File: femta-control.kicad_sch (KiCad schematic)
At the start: 13 parts, among them J2 CUBESAT INTERFACE, U4 LM358-N-Q1

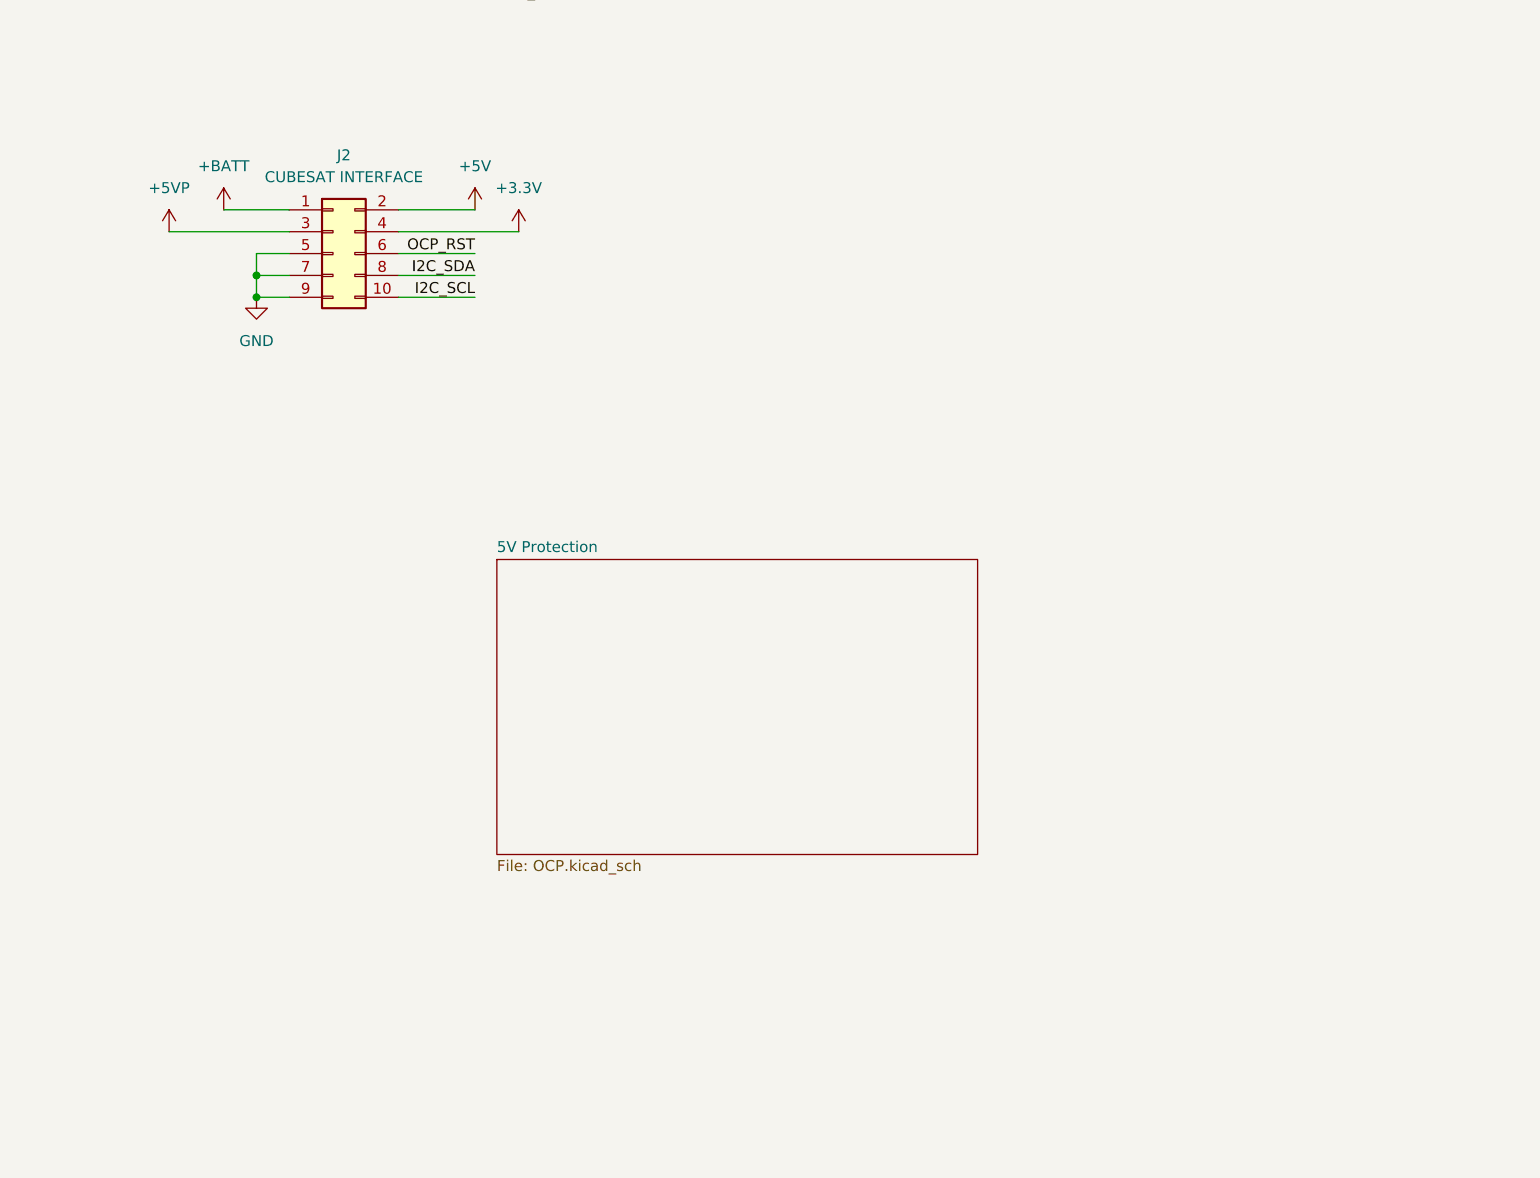
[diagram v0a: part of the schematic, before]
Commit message: ocp channels
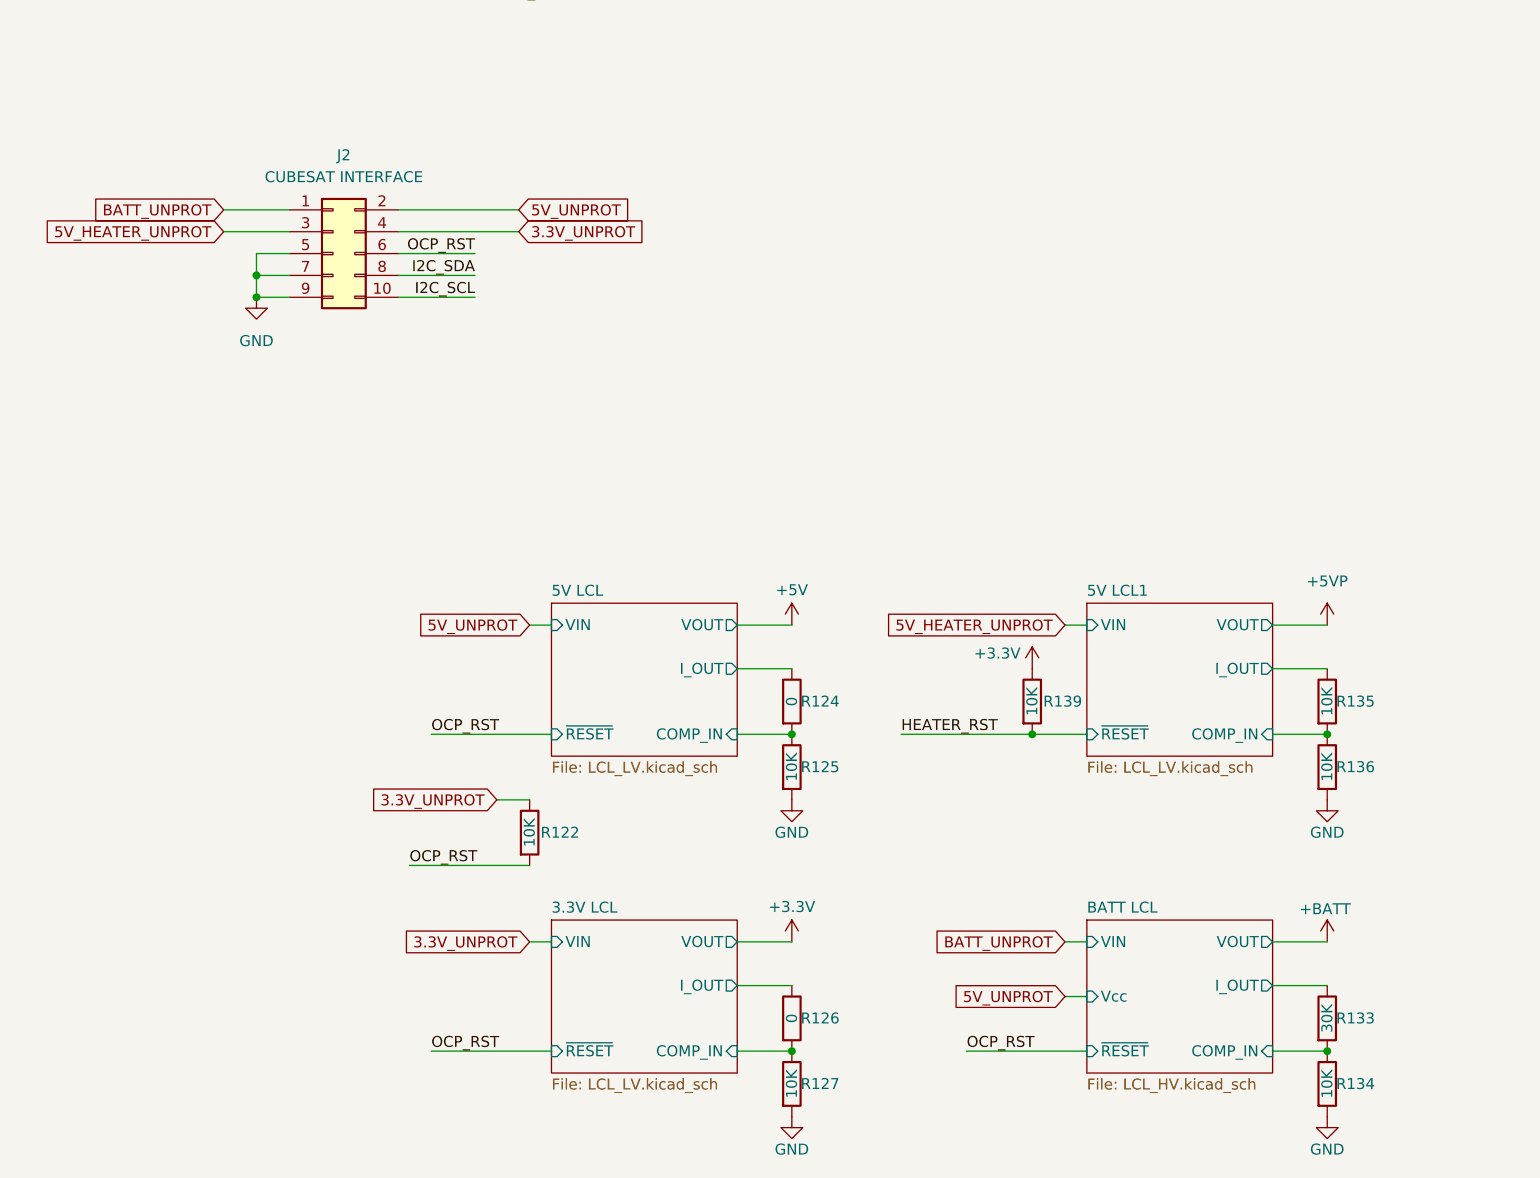
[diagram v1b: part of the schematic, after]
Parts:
- added R122, R125, R127, R134, R135, R136, R139: 10K, symbol Device:R
- added R124, R126: 0, symbol Device:R
- added R133: 30K, symbol Device:R
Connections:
- net +3.3V: now also R139.1; no longer J2.4 (Pin_4)
- net +5V: no longer J2.2 (Pin_2)
- net +5VP: no longer J2.3 (Pin_3)
- net +BATT: no longer J2.1 (Pin_1)
- net GND: now also R125.2, R127.2, R134.2, R136.2
- net OCP_RST: now also R122.2
- new net 3.3V LCL/COMP_IN: R126.2, R127.1
- new net 3.3V LCL/I_OUT: R126.1
- new net 3.3V_UNPROT: J2.4 (Pin_4), R122.1
- new net 5V LCL/COMP_IN: R124.2, R125.1
- new net 5V LCL/I_OUT: R124.1
- new net 5V LCL1/COMP_IN: R135.2, R136.1
- new net 5V LCL1/I_OUT: R135.1
- new net 5V_HEATER_UNPROT: J2.3 (Pin_3)
- new net 5V_UNPROT: J2.2 (Pin_2)
- new net BATT LCL/COMP_IN: R133.2, R134.1
- new net BATT LCL/I_OUT: R133.1
- new net BATT_UNPROT: J2.1 (Pin_1)
- new net HEATER_RST: R139.2
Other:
- removed sheet 5V Protection
- added sheet 3.3V LCL (LCL_LV.kicad_sch)
- added sheet 5V LCL (LCL_LV.kicad_sch)
- added sheet 5V LCL1 (LCL_LV.kicad_sch)
- added sheet BATT LCL (LCL_HV.kicad_sch)
